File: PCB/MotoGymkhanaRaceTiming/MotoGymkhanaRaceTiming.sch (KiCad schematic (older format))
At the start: 42 parts, among them U1 LM2577T-ADJ_NOPB, U2 PC817, U3 PC817

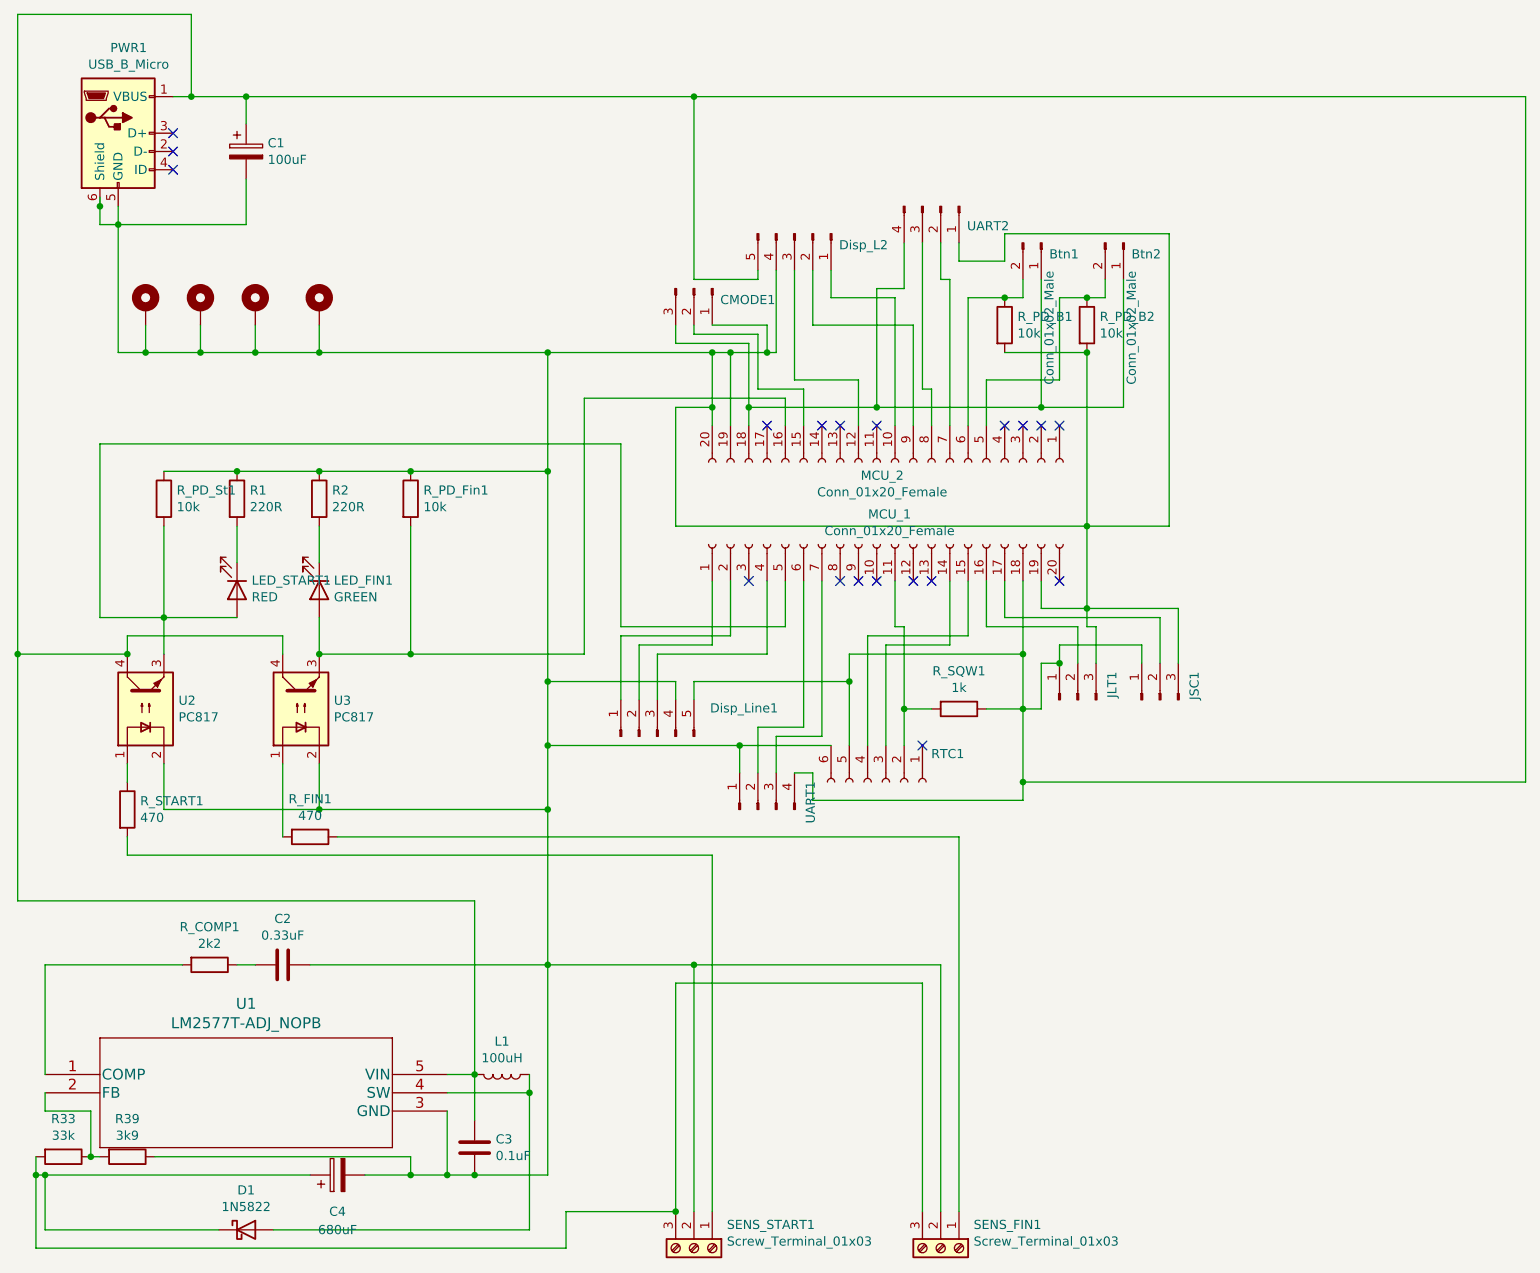
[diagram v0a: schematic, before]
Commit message: Schematic optimizations
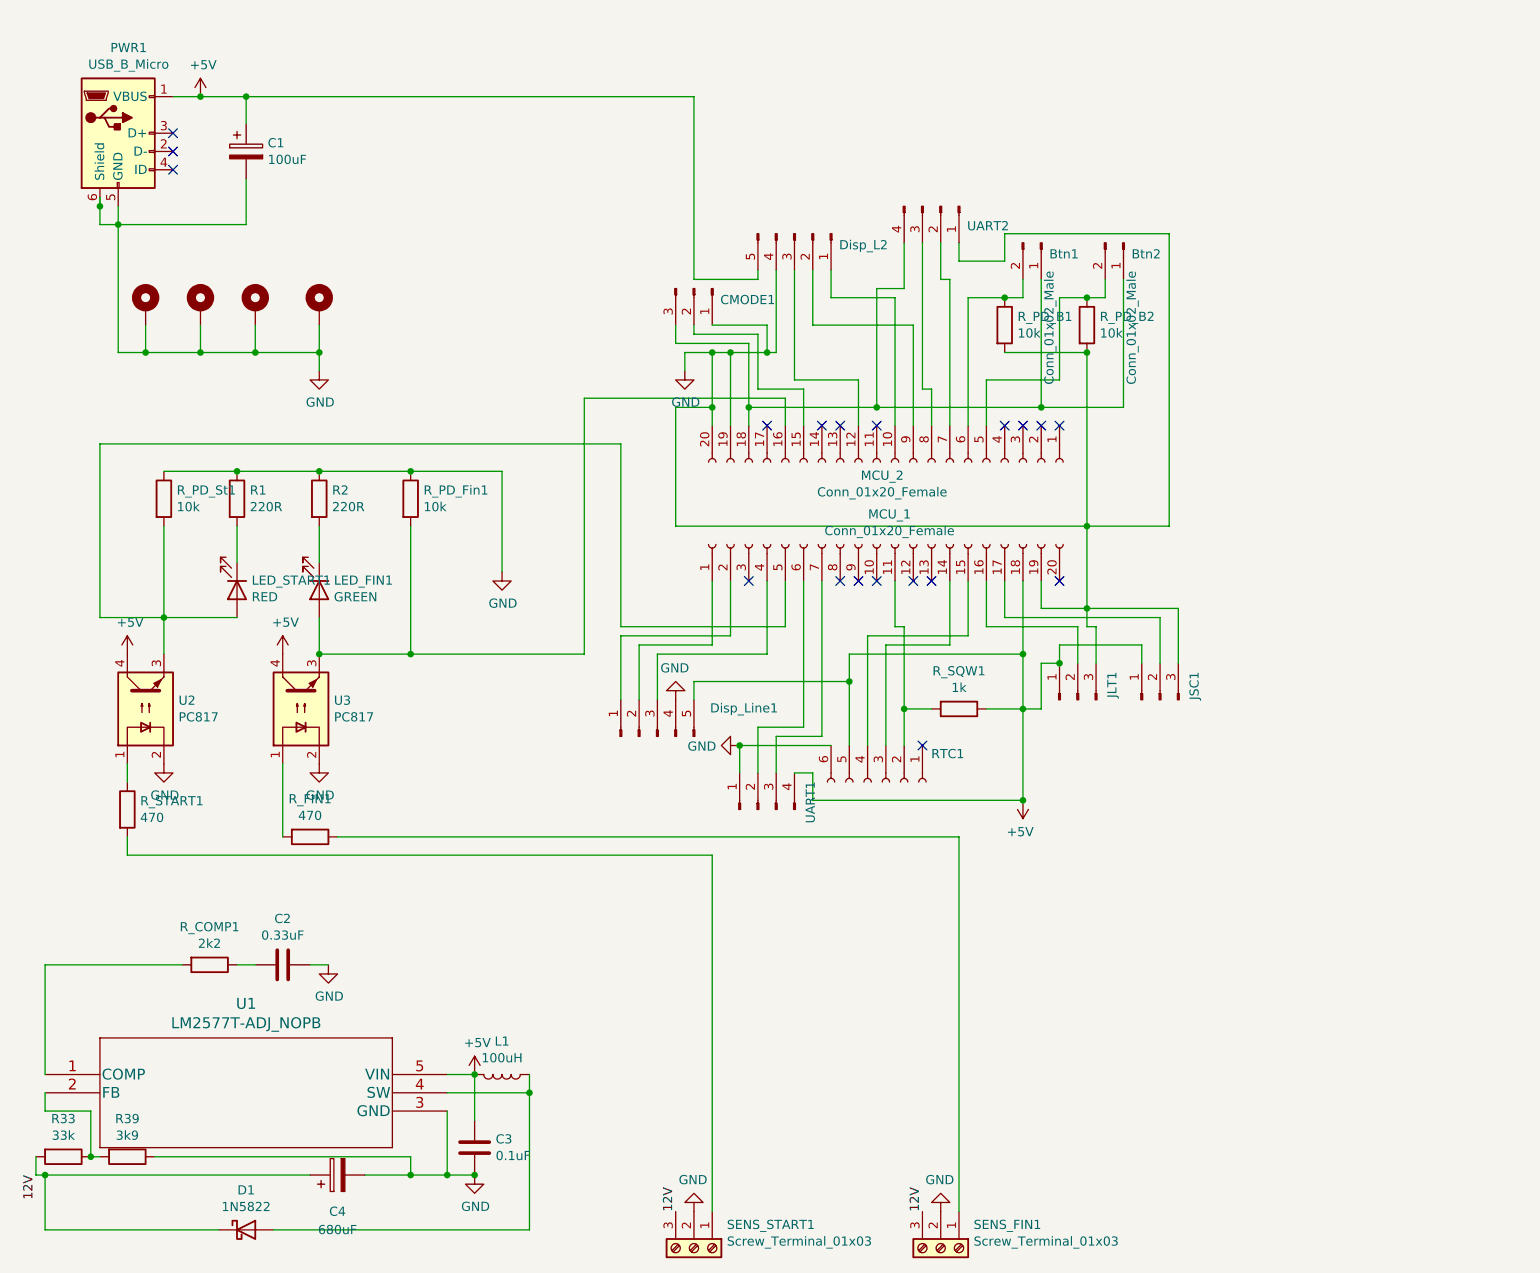
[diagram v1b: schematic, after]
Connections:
- net GND: now reaches C1.2, C2.1, C3.2, C4.2, CMODE1.1 (Pin_1), Disp_L2.4 (Pin_4), Disp_Line1.4 (Pin_4), H1.1, H2.1, H3.1, H4.1, JLT1.3 (Pin_3), JSC1.3 (Pin_3), MCU_1.19 (Pin_19), MCU_2.19 (Pin_19), MCU_2.20 (Pin_20), PWR1.5 (GND), PWR1.6 (Shield), R1.1, R2.1, R39.1, RTC1.6 (Pin_6), R_PD_B1.2, R_PD_B2.2, R_PD_Fin1.1, R_PD_St1.1, SENS_FIN1.2 (Pin_2), SENS_START1.2 (Pin_2), U1.3 (GND), U2.2, U3.2, UART1.1 (Pin_1), UART2.1 (Pin_1)
- net +5V: now reaches C1.1, C3.1, Disp_L2.5 (Pin_5), Disp_Line1.5 (Pin_5), JLT1.1 (Pin_1), JSC1.1 (Pin_1), L1.2, MCU_1.18 (Pin_18), PWR1.1 (VBUS), RTC1.5 (Pin_5), R_SQW1.1, U1.5 (VIN), U2.4, U3.4, UART1.4 (Pin_4)
- net 12V: now reaches C4.1, D1.1 (K), R33.2, SENS_FIN1.3 (Pin_3), SENS_START1.3 (Pin_3)
